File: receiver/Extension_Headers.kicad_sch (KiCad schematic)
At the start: 1 part, among them J2 Conn_02x05_Counter_Clockwise

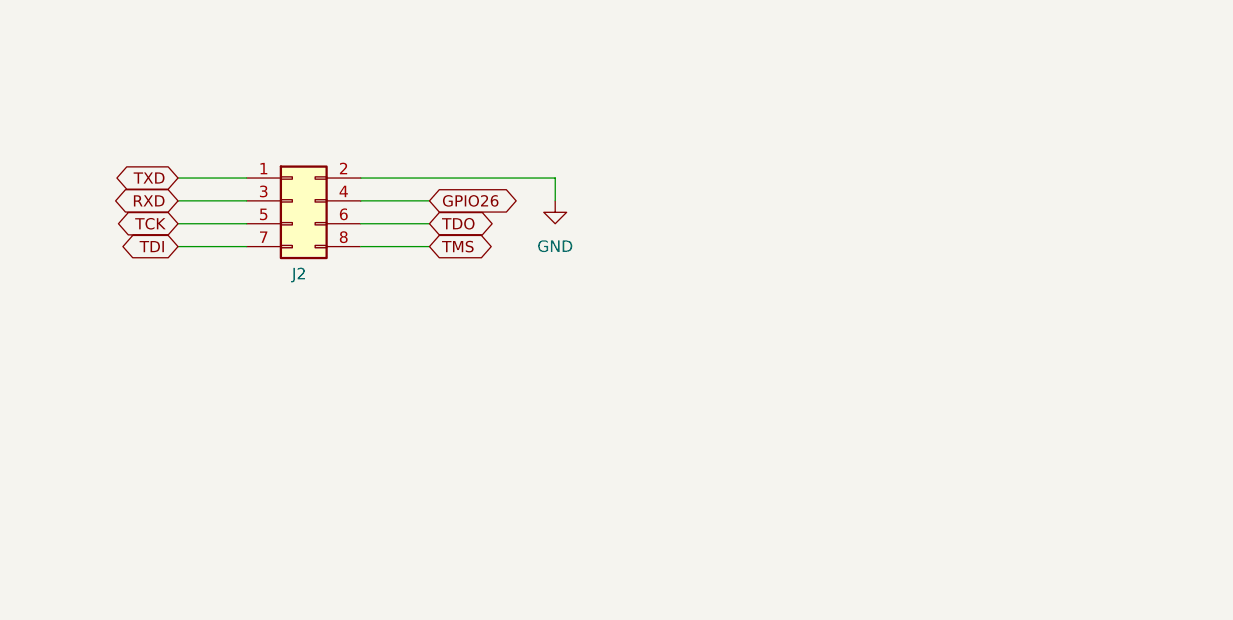
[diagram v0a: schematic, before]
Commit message: First draft of new board
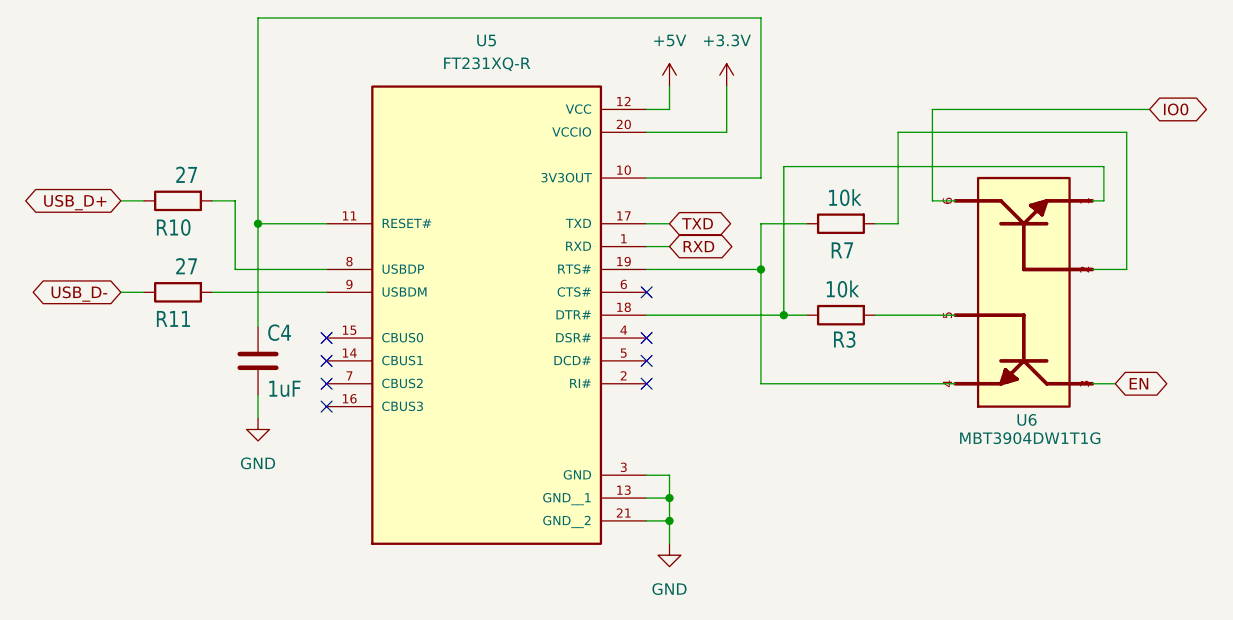
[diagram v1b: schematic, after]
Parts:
- removed J2: Conn_02x05_Counter_Clockwise, Connector_PinHeader_2.54mm:PinHeader_2x04_P2.54mm_Vertical, symbol Connector_Generic:Conn_02x04_Odd_Even
- added C4: 1uF, receiver:C0805, symbol Device:C
- added R10, R11: 27, Resistor_SMD:R_0805_2012Metric_Pad1.20x1.40mm_HandSolder, symbol Device:R
- added R3, R7: 10k, Resistor_SMD:R_0805_2012Metric_Pad1.20x1.40mm_HandSolder, symbol Device:R
- added U5: FT231XQ-R, FT231XQ-R:QFN50P400X400X80-21N, symbol receiver:FT231XQ-R
- added U6: MBT3904DW1T1G, MBT3904DW1T1G:SOT236, symbol receiver:MBT3904DW1T1G
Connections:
- net GND: now also C4.2, U5.13 (GND__1), U5.21 (GND__2), U5.3 (GND)
- net RXD: now also U5.1 (RXD)
- net TXD: now also U5.17 (TXD)
- new net: R7.1, U5.19 (RTS#), U6.4
- new net: R7.2, U6.2
- new net: C4.1, U5.10 (3V3OUT), U5.11 (RESET#)
- new net: R10.2, U5.8 (USBDP)
- new net: R3.1, U5.18 (DTR#), U6.1
- new net: R3.2, U6.5
- new net: R11.2, U5.9 (USBDM)
- new net +3.3V: U5.20 (VCCIO)
- new net +5V: U5.12 (VCC)
- new net EN: U6.3
- new net IO0: U6.6
- new net USB_D+: R10.1
- new net USB_D-: R11.1
- no-connect marks 0 -> 8
